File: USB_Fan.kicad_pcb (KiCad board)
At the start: 4 copper layers, 36.4 x 25.7 mm, 38 parts, among them J1 USB-C (Female), J2 Fan, J3 Fan Voltage, SW1 Power, U1 TP4056, U2 DW01A-G, U3 FS8205A, U4 TPS61170

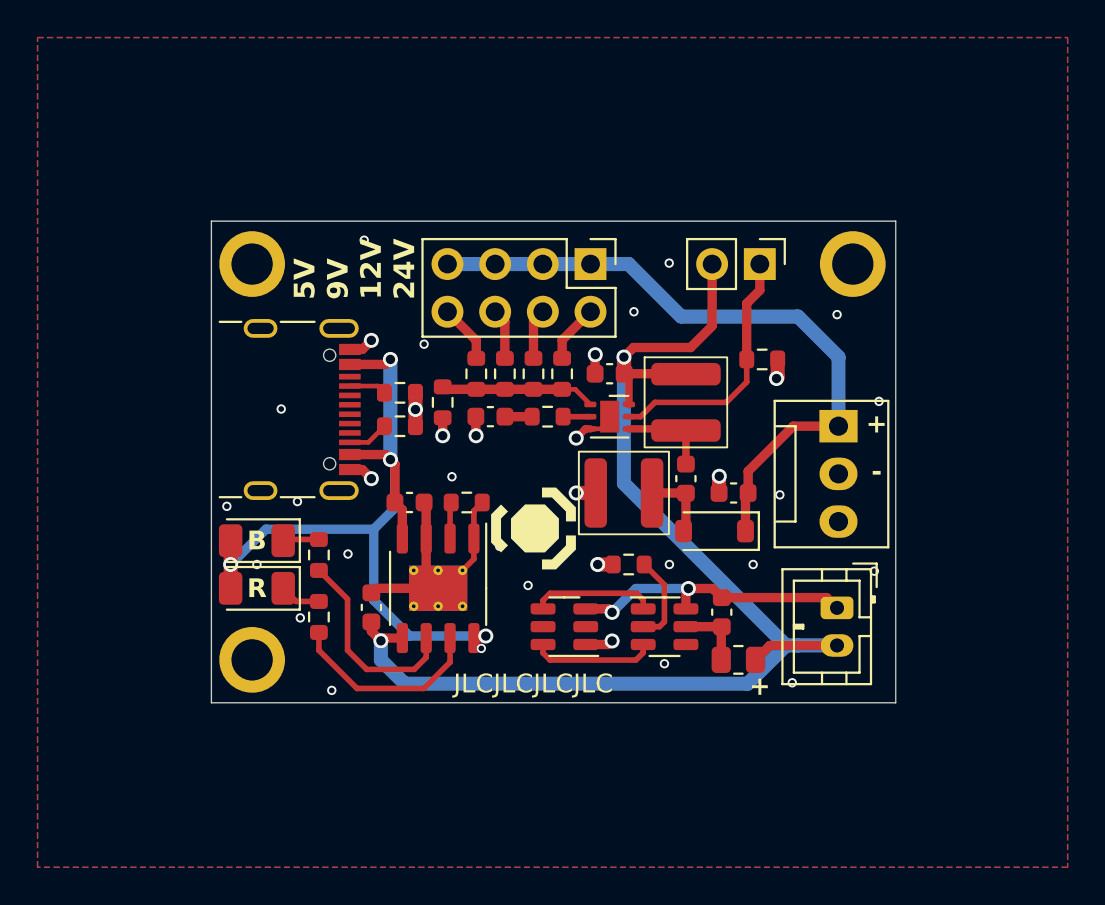
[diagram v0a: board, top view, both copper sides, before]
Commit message: Fix problems on the PCB
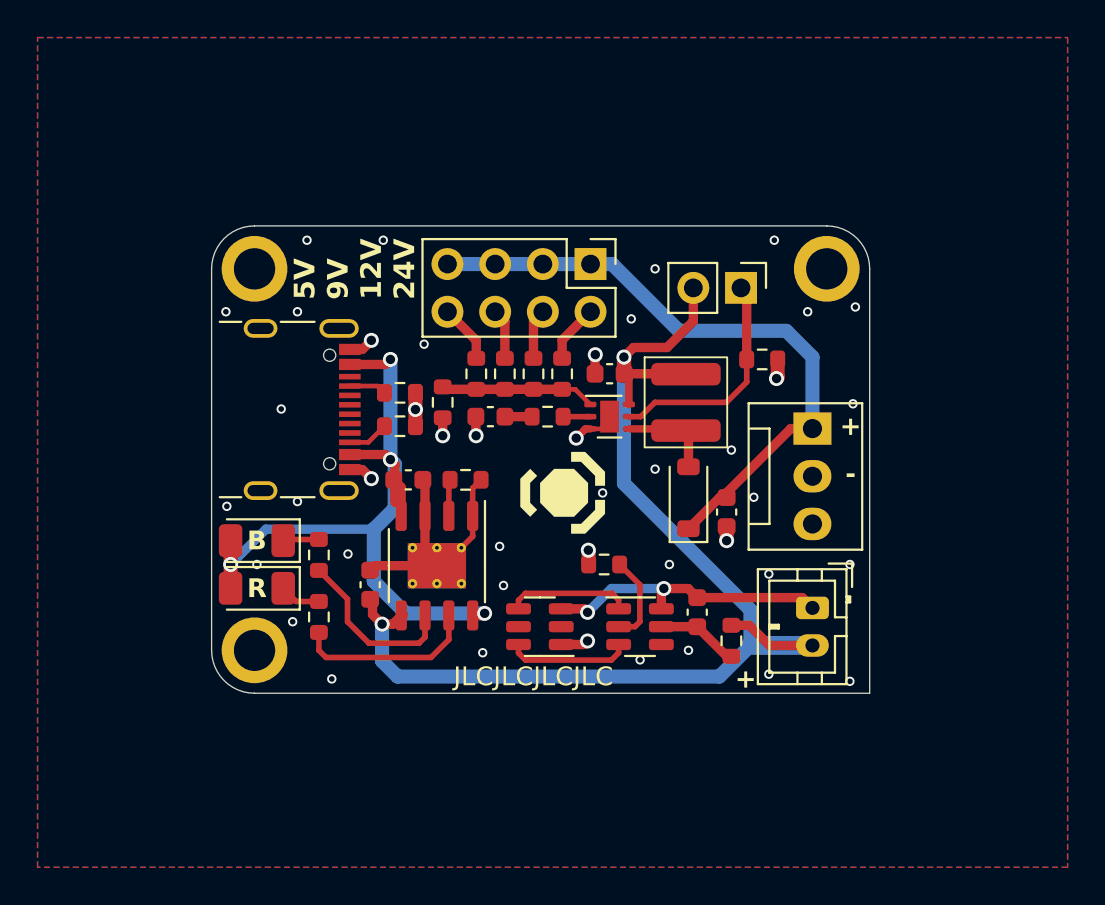
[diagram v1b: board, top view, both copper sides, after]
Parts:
- removed the C6 at (103.7, 50.8)
- removed L2: 10uH, Custom:Inductor 4x4
- R7: footprint Resistor_SMD:R_0805_2012Metric -> Resistor_SMD:R_0603_1608Metric
- moved D1 2.26 mm to (103.9, 51.8), turned to 90 degrees
- moved SW1 1.62 mm to (106.7, 40.6)
- moved H4 1.41 mm to (111.3, 39.6)
- moved J2 1.39 mm to (110.5, 48.1)
- moved BT1 1.31 mm to (110.5, 57.7)
- moved U3 1.31 mm to (96.0, 58.7)
- moved C3 1.31 mm to (104.4, 57.9)
- moved R6 1.31 mm to (99.4, 55.4)
- moved U2 1.31 mm to (101.3, 58.7)
- moved U1 1.21 mm to (90.5, 55.4)
- moved C1 1.21 mm to (89.0, 50.9)
- moved C2 1.21 mm to (86.9, 56.5)
- moved R5 1.21 mm to (92.0, 50.9)
- moved C6 1.08 mm to (105.9, 52.6), turned to -90 degrees
- moved R7 1.08 mm to (106.2, 59.4), turned to 90 degrees
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- renumbered C7 to C6
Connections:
- L1 pad 2: Net-(U4-SW) -> Net-(D1-A)
- U4 pad 4: Net-(U4-SW) -> Net-(D1-A)
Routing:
- net Net-(U4-SW): track 4.86 -> 0.00 mm
- net +BATT: track 67.3 -> 63.9 mm
- net /Standby: track 10.8 -> 9.25 mm
- net Net-(SW1-A): track 13.6 -> 12.2 mm
- net /V_{OUT}: track 35.6 -> 34.3 mm
- net GND: track 27.8 -> 26.6 mm, vias 35 -> 43
- net Net-(D1-A): track 3.88 -> 5.06 mm
- net +5V: track 40.8 -> 39.6 mm
- net /Charging: track 10.6 -> 9.71 mm
- net /DW01A Vcc: track 3.69 -> 4.38 mm
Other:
- board size 36.4 x 25.7 mm -> 35.1 x 24.9 mm
